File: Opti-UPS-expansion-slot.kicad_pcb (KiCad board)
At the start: 2 copper layers, 205.7 x 71.1 mm, 36 parts, among them J1 Expansion_Slot_Ribbon_Connect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, J11 I2C Header, J12 I2C Header, J2 M3-Screw-Terminal-90, J3 M3-Screw-Terminal-90, J4 Expansion_Slot_Ribbon_Connect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, J5 M3-Screw-Terminal-90, J6 M3-Screw-Terminal-90, Q1 BC557, Q3 BC557, U1 MP4560_Regulator_Module, U2 MAX3232_Module, U3 RockPi-S, U4 MP4560_Regulator_Module, U5 MAX3232_Module, U6 orange_pi_zero

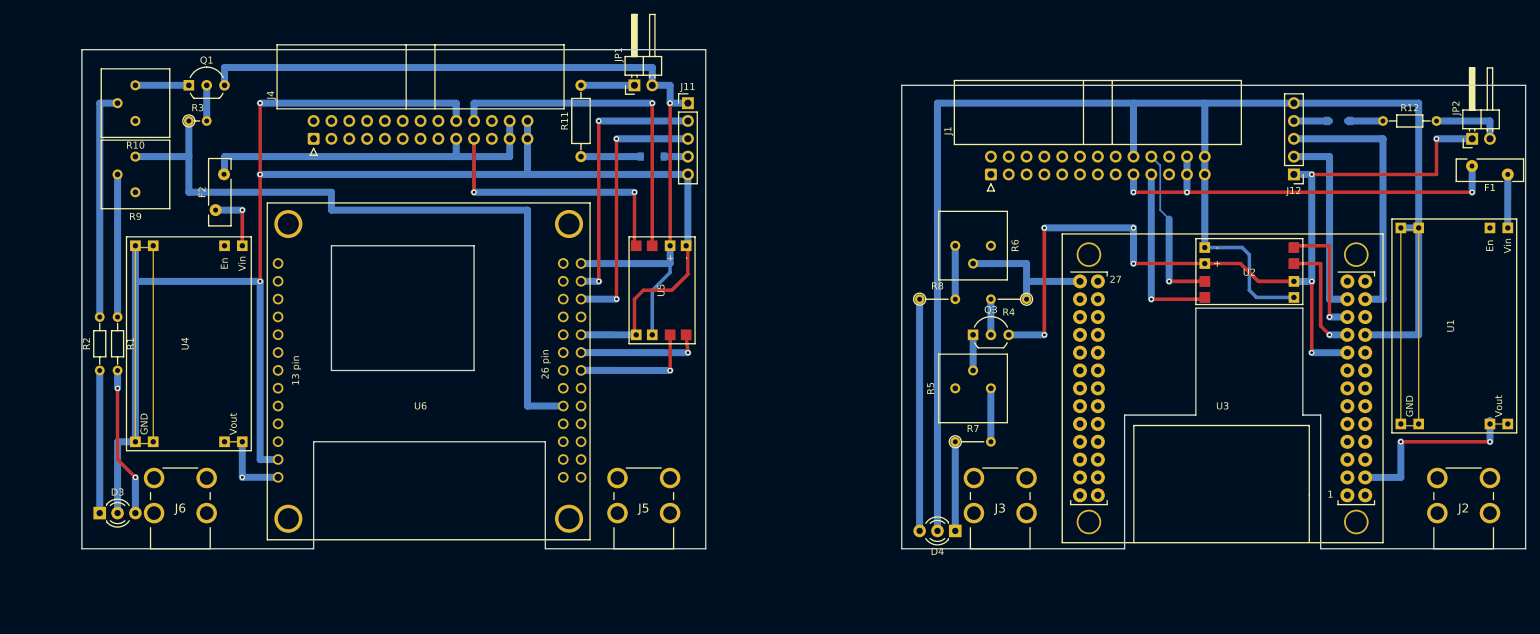
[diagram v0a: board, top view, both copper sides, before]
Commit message: revision 1.1
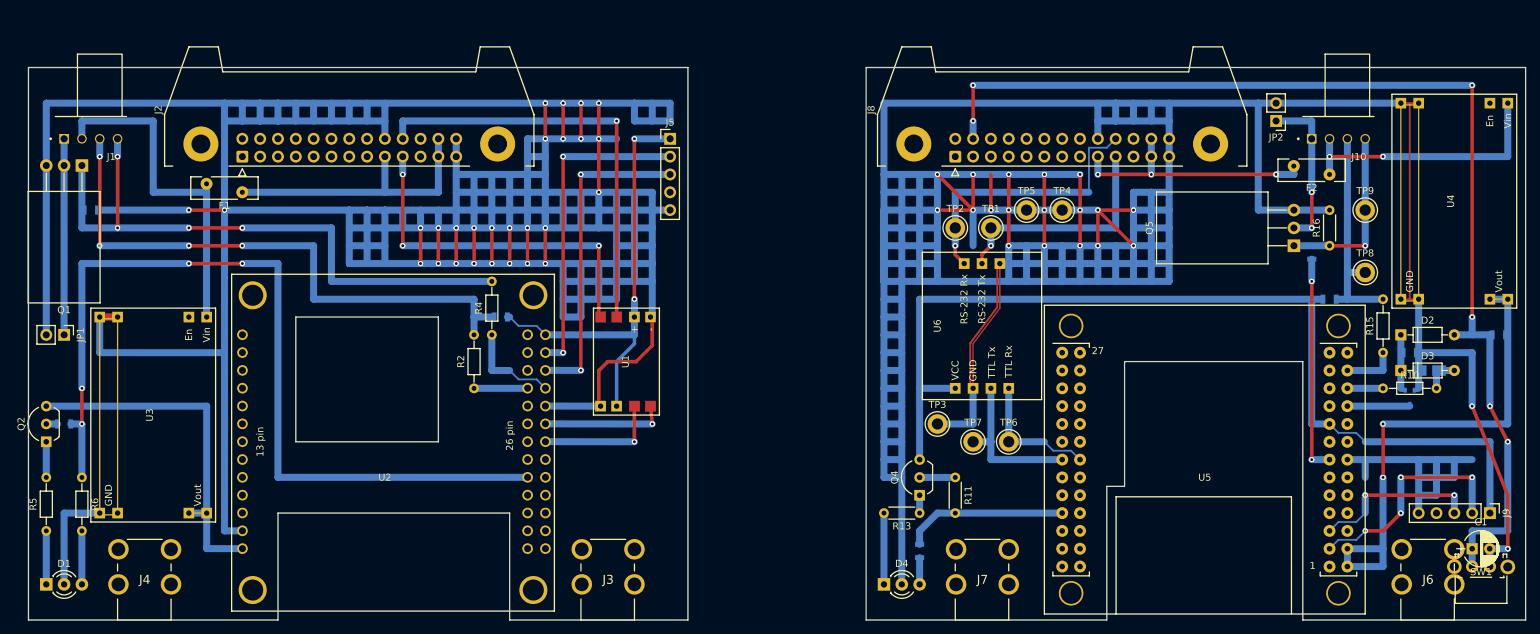
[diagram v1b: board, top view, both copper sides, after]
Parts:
- removed D5, D6: B0520LW, Diodes_SMD:D_SOD-123
- removed J11, J12: I2C Header, Pin_Headers:Pin_Header_Straight_1x05_Pitch2.54mm
- removed the J4 at (76.2, 78.7)
- removed the R5 at (172.7, 114.3)
- removed the R6 at (167.6, 94.0)
- removed the U1 at (246.4, 91.4)
- added C1: 1uF, Opti-UPS Expansion Slot:CP_Radial_D5.0mm_P2.50mm, F.Cu at (241.3, 137.2)
- added C2: 47uF, Opti-UPS Expansion Slot:CP_Tantalum_Case-A_EIA-3216-18_Reflow, B.Cu at (235.2, 111.8)
- added D2: BAT43, Opti-UPS Expansion Slot:D_DO-35_SOD27_P7.62mm_Horizontal, F.Cu at (231.1, 106.7)
- added D3: BAT43, Opti-UPS Expansion Slot:D_DO-35_SOD27_P7.62mm_Horizontal, F.Cu at (231.1, 111.8)
- added J10: PWM Fan, Opti-UPS Expansion Slot:Fan_Pin_Header_4Pin_Horizontal, F.Cu at (218.4, 78.7)
- added J2: Expansion_Slot_Ribbon_Connector, Opti-UPS Expansion Slot:IDC-Header_2x13-1MP_P2.54mm_Latch_Horizontal, F.Cu at (66.0, 81.3)
- added J5: I2C Header, Opti-UPS Expansion Slot:Pin_Header_Straight_1x05_Pitch2.54mm, F.Cu at (127.0, 78.7)
- added J8: Expansion_Slot_Ribbon_Connector, Opti-UPS Expansion Slot:IDC-Header_2x13-1MP_P2.54mm_Latch_Horizontal, F.Cu at (167.6, 81.3)
- added J9: I2C Header, Opti-UPS Expansion Slot:Pin_Header_Straight_1x05_Pitch2.54mm, F.Cu at (243.8, 132.1)
- added Q1: IRFZ44N, Opti-UPS Expansion Slot:TO-220-3_Horizontal, F.Cu at (43.2, 82.5)
- added Q4: BC557, Opti-UPS Expansion Slot:TO-92_Inline_Wide, F.Cu at (162.6, 129.5)
- added Q5: IRLZ44N, Opti-UPS Expansion Slot:TO-220-3_Horizontal, F.Cu at (215.9, 94.0)
- added R1: 2k2, Opti-UPS Expansion Slot:R_0805, B.Cu at (102.9, 104.1)
- added R14: 2k2, Opti-UPS Expansion Slot:R_0805, B.Cu at (221.0, 101.6)
- added R15: 47, Opti-UPS Expansion Slot:R_Axial_DIN0204_L3.6mm_D1.6mm_P7.62mm_Horizontal, F.Cu at (228.6, 109.2)
- added R16: 10k, Opti-UPS Expansion Slot:R_Axial_DIN0204_L3.6mm_D1.6mm_P5.08mm_Horizontal, F.Cu at (221.0, 94.0)
- added R17: 47, Opti-UPS Expansion Slot:R_0805, B.Cu at (218.4, 94.9)
- added R2: 50, Opti-UPS Expansion Slot:R_Axial_DIN0204_L3.6mm_D1.6mm_P7.62mm_Horizontal, F.Cu at (99.1, 114.3)
- added R3: 10k, Opti-UPS Expansion Slot:R_0805, B.Cu at (44.5, 88.9)
- added SW1: SW_Push, Opti-UPS Expansion Slot:SW_Tactile_SPST_Angled_PTS645Vx83-2LFS, F.Cu at (243.8, 139.7)
- added TP1: TestPoint, Opti-UPS Expansion Slot:Test_Point_Keystone_Yellow, F.Cu at (172.7, 91.4)
- added TP2: TestPoint, Opti-UPS Expansion Slot:Test_Point_Keystone_Green, F.Cu at (167.6, 91.4)
- added TP3: TestPoint, Opti-UPS Expansion Slot:Test_Point_Keystone_Black, F.Cu at (165.1, 119.4)
- added TP4: TestPoint, Opti-UPS Expansion Slot:Test_Point_Keystone_Black, F.Cu at (182.9, 88.9)
- added TP5: TestPoint, Opti-UPS Expansion Slot:Test_Point_Keystone_Black, F.Cu at (177.8, 88.9)
- added TP6: TestPoint, Opti-UPS Expansion Slot:Test_Point_Keystone_Green, F.Cu at (175.3, 121.9)
- added TP7: TestPoint, Opti-UPS Expansion Slot:Test_Point_Keystone_Yellow, F.Cu at (170.2, 121.9)
- added TP8: TestPoint, Opti-UPS Expansion Slot:Test_Point_Keystone_White, F.Cu at (226.1, 97.8)
- added TP9: TestPoint, Opti-UPS Expansion Slot:Test_Point_Keystone_Blue, F.Cu at (226.1, 88.9)
- added U3: MP4560_Regulator_Module, Opti-UPS Expansion Slot:MP4560_Regulator_Module, F.Cu at (61.0, 104.1)
- D1: renamed from D3; footprint LEDs:LED_D3.0mm-3 -> Opti-UPS Expansion Slot:LED_D3.0mm-3
- D4: footprint LEDs:LED_D3.0mm-3 -> Opti-UPS Expansion Slot:LED_D3.0mm-3
- F1: value 1-2A -> 0.5-1A; footprint Fuse:Fuse_Bourns_MF-RHT200 -> Opti-UPS Expansion Slot:Fuse_Bourns_MF-RHT200
- F2: value 0.5-1A -> 1-2A; footprint Fuse:Fuse_Bourns_MF-RHT200 -> Opti-UPS Expansion Slot:Fuse_Bourns_MF-RHT200
- J1: value Expansion_Slot_Ribbon_Connector -> PWM Fan; footprint Connector_IDC:IDC-Header_2x13_P2.54mm_Horizontal -> Opti-UPS Expansion Slot:Fan_Pin_Header_4Pin_Horizontal
- J3: renamed from J5; footprint moonbuggy-custom:M3-Screw-Terminal-90 -> Opti-UPS Expansion Slot:M3-Screw-Terminal-90
- J4: renamed from J6; footprint moonbuggy-custom:M3-Screw-Terminal-90 -> Opti-UPS Expansion Slot:M3-Screw-Terminal-90
- J6: renamed from J2; footprint moonbuggy-custom:M3-Screw-Terminal-90 -> Opti-UPS Expansion Slot:M3-Screw-Terminal-90
- J7: renamed from J3; footprint moonbuggy-custom:M3-Screw-Terminal-90 -> Opti-UPS Expansion Slot:M3-Screw-Terminal-90
- JP1, JP2: value Jumper_NO_Small -> Jumper_2_Open; footprint Pin_Headers:Pin_Header_Angled_1x02_Pitch2.54mm -> Opti-UPS Expansion Slot:Pin_Header_Straight_1x02_Pitch2.54mm
- Q2: renamed from Q1; footprint TO_SOT_Packages_THT:TO-92_Inline_Wide -> Opti-UPS Expansion Slot:TO-92_Inline_Wide
- Q3: value BC557 -> SM3K102TU; footprint TO_SOT_Packages_THT:TO-92_Inline_Wide -> Opti-UPS Expansion Slot:SOT-323_SC-70; moved to B.Cu
- R10: value 1k -> 1k5; footprint Potentiometer_THT:Potentiometer_Bourns_3386P_Vertical -> Opti-UPS Expansion Slot:R_Axial_DIN0204_L3.6mm_D1.6mm_P7.62mm_Horizontal
- R11: value 20 -> 15k; footprint Resistors_THT:R_Axial_DIN0207_L6.3mm_D2.5mm_P10.16mm_Horizontal -> Opti-UPS Expansion Slot:R_Axial_DIN0204_L3.6mm_D1.6mm_P5.08mm_Horizontal
- R12: value 20 -> 750; footprint Resistors_THT:R_Axial_DIN0204_L3.6mm_D1.6mm_P7.62mm_Horizontal -> Opti-UPS Expansion Slot:R_0805; moved to B.Cu
- R13: renamed from R7; value 75 -> 750; footprint Resistors_THT:R_Axial_DIN0204_L3.6mm_D1.6mm_P5.08mm_Vertical -> Opti-UPS Expansion Slot:R_Axial_DIN0204_L3.6mm_D1.6mm_P5.08mm_Horizontal
- R4: value 15k -> 50; footprint Resistors_THT:R_Axial_DIN0204_L3.6mm_D1.6mm_P5.08mm_Vertical -> Opti-UPS Expansion Slot:R_Axial_DIN0204_L3.6mm_D1.6mm_P7.62mm_Horizontal
- R5: renamed from R2; value 75 -> 1k5; footprint Resistors_THT:R_Axial_DIN0204_L3.6mm_D1.6mm_P7.62mm_Horizontal -> Opti-UPS Expansion Slot:R_Axial_DIN0204_L3.6mm_D1.6mm_P7.62mm_Horizontal
- R6: renamed from R1; value 75 -> 1k5; footprint Resistors_THT:R_Axial_DIN0204_L3.6mm_D1.6mm_P7.62mm_Horizontal -> Opti-UPS Expansion Slot:R_Axial_DIN0204_L3.6mm_D1.6mm_P7.62mm_Horizontal
- R7: renamed from R3; footprint Resistors_THT:R_Axial_DIN0204_L3.6mm_D1.6mm_P2.54mm_Vertical -> Opti-UPS Expansion Slot:R_0805; moved to B.Cu
- R8: value 75 -> 15k; footprint Resistors_THT:R_Axial_DIN0204_L3.6mm_D1.6mm_P5.08mm_Vertical -> Opti-UPS Expansion Slot:R_0805; moved to B.Cu
- R9: value 1k -> 1M; footprint Potentiometer_THT:Potentiometer_Bourns_3386P_Vertical -> Opti-UPS Expansion Slot:R_0805; moved to B.Cu
- U1: renamed from U5; footprint moonbuggy-custom:MAX3232_Module -> Opti-UPS Expansion Slot:MAX3232_Module
- U2: value MAX3232_Module -> orange_pi_zero; footprint moonbuggy-custom:MAX3232_Module -> Opti-UPS Expansion Slot:orangepi-zero-headers-no-debug
- U4: footprint Custom:MP4560_Regulator_Module -> Opti-UPS Expansion Slot:MP4560_Regulator_Module
- U5: renamed from U3; footprint RockPi:RockPi-S-pads-only -> Opti-UPS Expansion Slot:RockPi-S-pads-only
- U6: value orange_pi_zero -> SP3232_Module; footprint orangepi-zero:orangepi-zero-headers-no-debug -> Opti-UPS Expansion Slot:SP3232_Module_1CH
- moved R9 183.7 mm to (232.4, 109.2), turned to 0 degrees
- moved R10 183.0 mm to (228.6, 114.3), turned to 0 degrees
- moved U4 181.5 mm to (246.4, 73.7)
- moved F1 180.4 mm to (66.0, 86.4)
- moved F2 158.8 mm to (221.0, 83.8), turned to 180 degrees
- moved J1 132.2 mm to (40.6, 78.7), turned to 180 degrees
- moved U2 109.6 mm to (106.7, 106.7)
- moved R12 90.1 mm to (162.6, 137.5), turned to 270 degrees
- moved JP1 88.7 mm to (40.6, 106.7), turned to 270 degrees
- moved R8 82.7 mm to (245.1, 106.7), turned to 180 degrees
- moved R4 76.4 mm to (101.6, 106.7), turned to 90 degrees
- moved R11 70.3 mm to (167.6, 127.0), turned to 270 degrees
- moved Q3 62.9 mm to (232.4, 115.6), turned to 270 degrees
- moved U6 59.3 mm to (170.2, 106.7), turned to 90 degrees
- moved Q2 54.7 mm to (38.1, 121.9), turned to 90 degrees
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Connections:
- net Net-(F2-Pad1) renamed RPiS-12V-fused
- F1 pad 1: Net-(F1-Pad1) -> +12V
- F1 pad 2: +12V -> OPiZ-12V-fused
- J1 pad 1: (no net) -> Net-(J1-Pad1)
- J1 pad 2: (no net) -> OPiZ-12V-fused
- J1 pad 3: (no net) -> /Orange Pi Zero/tacho
- J1 pad 4: (no net) -> /Orange Pi Zero/PWM
- JP1 pad 1: Net-(JP1-Pad1) -> Net-(J1-Pad1)
- JP1 pad 2: /Orange Pi Zero/3.3v -> GND
- JP2 pad 1: /Rock Pi S/3.3v -> /Rock Pi S/FAN_GND
- JP2 pad 2: Net-(JP2-Pad2) -> GND
- Q2 pad 1: Net-(Q1-Pad1) -> Net-(Q2-Pad1)
- Q2 pad 3: /Orange Pi Zero/3.3v -> OPiZ-5V
- Q3 pad 1: Net-(Q3-Pad1) -> Net-(D2-Pad1)
- Q3 pad 2: Net-(Q3-Pad2) -> GND
- Q3 pad 3: /Rock Pi S/3.3v -> Net-(Q3-Pad3)
- R10 pad 1: Net-(Q1-Pad1) -> Net-(R10-Pad1)
- R10 pad 2: Net-(R10-Pad2) -> Net-(C2-Pad1)
- R11 pad 2: Net-(JP1-Pad1) -> /Rock Pi S/GPIO_ready
- R12 pad 1: Net-(D6-Pad2) -> /Rock Pi S/GPIO_ready
- R12 pad 2: Net-(JP2-Pad2) -> /Rock Pi S/green
- R13 pad 1: /Rock Pi S/red -> Net-(Q4-Pad1)
- R13 pad 2: Net-(R5-Pad1) -> /Rock Pi S/red
- R4 pad 1: Net-(R4-Pad1) -> OPiZ-Fan-PWM
- R4 pad 2: Net-(Q3-Pad2) -> /Orange Pi Zero/PWM
- R5 pad 2: Net-(R10-Pad2) -> Net-(Q2-Pad1)
- R6 pad 1: Net-(R1-Pad1) -> /Orange Pi Zero/GPIO_ready
- R7 pad 1: Net-(R3-Pad1) -> /Orange Pi Zero/GPIO_ready
- R8 pad 1: /Rock Pi S/green -> RPiS-5V
- R9 pad 1: Net-(R3-Pad1) -> Net-(D2-Pad1)
- R9 pad 2: Net-(R1-Pad1) -> GND
- U1 pad 2: /Orange Pi Zero/3.3v -> OPiZ-3V3
- U1 pad 6: /Orange Pi Zero/3.3v -> OPiZ-3V3
- U2 pad 1: GND -> OPiZ-5V
- U2 pad 2: /Rock Pi S/3.3v -> GND
- U2 pad 3: /Rock Pi S/TTL-Tx -> (no net)
- U2 pad 4: /Rock Pi S/TTL-Rx -> (no net)
- U2 pad 5: GND -> (no net)
- U2 pad 6: /Rock Pi S/3.3v -> (no net)
- U2 pad 7: /Rock Pi S/RS232-Tx -> (no net)
- U2 pad 8: /Rock Pi S/RS232-Rx -> (no net)
- U4 pad 7: /Orange Pi Zero/5V -> RPiS-5V
- U4 pad 8: /Orange Pi Zero/5V -> RPiS-5V
- U5 pad 13: (no net) -> RPiS-Fan-PWM
- U5 pad 14: (no net) -> RPiS-I2C-GND
- U5 pad 17: /Rock Pi S/3.3v -> +3V3
- U5 pad 19: /Rock Pi S/TTL-Tx -> (no net)
- U5 pad 2: (no net) -> RPiS-5V
- U5 pad 20: GND -> Net-(Q3-Pad3)
- U5 pad 21: /Rock Pi S/TTL-Rx -> (no net)
- U5 pad 22: (no net) -> Net-(R10-Pad1)
- U5 pad 23: /Rock Pi S/SDA -> (no net)
- U5 pad 24: /Rock Pi S/SCL -> RPiS-Fan-Tacho
- U5 pad 28: Net-(R4-Pad1) -> (no net)
- U5 pad 3: (no net) -> /Rock Pi S/SDA
- U5 pad 39: (no net) -> RPiS-TTL-Tx
- U5 pad 4: /Rock Pi S/5V -> RPiS-5V
- U5 pad 40: (no net) -> RPiS-TTL-Rx
- U5 pad 46: (no net) -> /Rock Pi S/GPIO_ready
- U5 pad 5: (no net) -> /Rock Pi S/SCL
- U6 pad 1: /Orange Pi Zero/5V -> +3V3
- U6 pad 3: (no net) -> RPiS-TTL-Rx
- U6 pad 4: (no net) -> RPiS-TTL-Tx
- U6 pad 5: (no net) -> GND
- U6 pad 6: (no net) -> /Rock Pi S/RS232-Rx
- U6 pad 7: (no net) -> /Rock Pi S/RS232-Tx
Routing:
- net GND: track 466.9 -> 1582.5 mm, vias 3 -> 47
- net Net-(C1-Pad1): track 7.62 -> 158.1 mm, vias 0 -> 6
- net +3V3: track 0.00 -> 139.5 mm
- net /Orange Pi Zero/GPIO_ready: track 0.00 -> 126.1 mm, vias 0 -> 4
- net /Rock Pi S/3.3v: track 125.5 -> 0.00 mm, vias 8 -> 0
- net /Orange Pi Zero/3.3v: track 120.4 -> 0.00 mm, vias 1 -> 0
- net Net-(R3-Pad1): track 101.6 -> 0.00 mm
- net /Orange Pi Zero/PWM: track 0.00 -> 87.6 mm, vias 0 -> 4
- net /Orange Pi Zero/tacho: track 0.00 -> 83.8 mm, vias 0 -> 4
- net RPiS-5V: track 0.00 -> 71.1 mm, vias 0 -> 2
- net OPiZ-3V3: track 0.00 -> 63.4 mm, vias 0 -> 2
- net OPiZ-5V: track 0.00 -> 50.8 mm
- net OPiZ-12V-fused: track 0.00 -> 49.5 mm
- net RPiS-I2C-GND: track 0.00 -> 43.2 mm
- net Net-(R10-Pad2): track 33.0 -> 0.00 mm
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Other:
- board size 205.7 x 71.1 mm -> 213.4 x 78.7 mm
- board text added: "35"
- board text added: "36"
- board text removed: "2"
- board text removed: "27"
- board text removed: "3"
- board text removed: "34"
- board text removed: "4"
